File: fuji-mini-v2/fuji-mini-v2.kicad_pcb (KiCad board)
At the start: 2 copper layers, 58.4 x 81.3 mm, 59 parts, among them J1 Micro_SD_Card, J2 AudioJack3_SwitchT, J4 USB_C_Receptacle_USB2.0_14P, SW1 RotaryEncoder_Switch, U1 ESP32-S3, U2 PCM5102A, U3 TPA6110A2DGN, U4 ER_OLEDM0.91_1x-I2C, U5 MCP73831-2-MC, U6 AMS1117-3.3

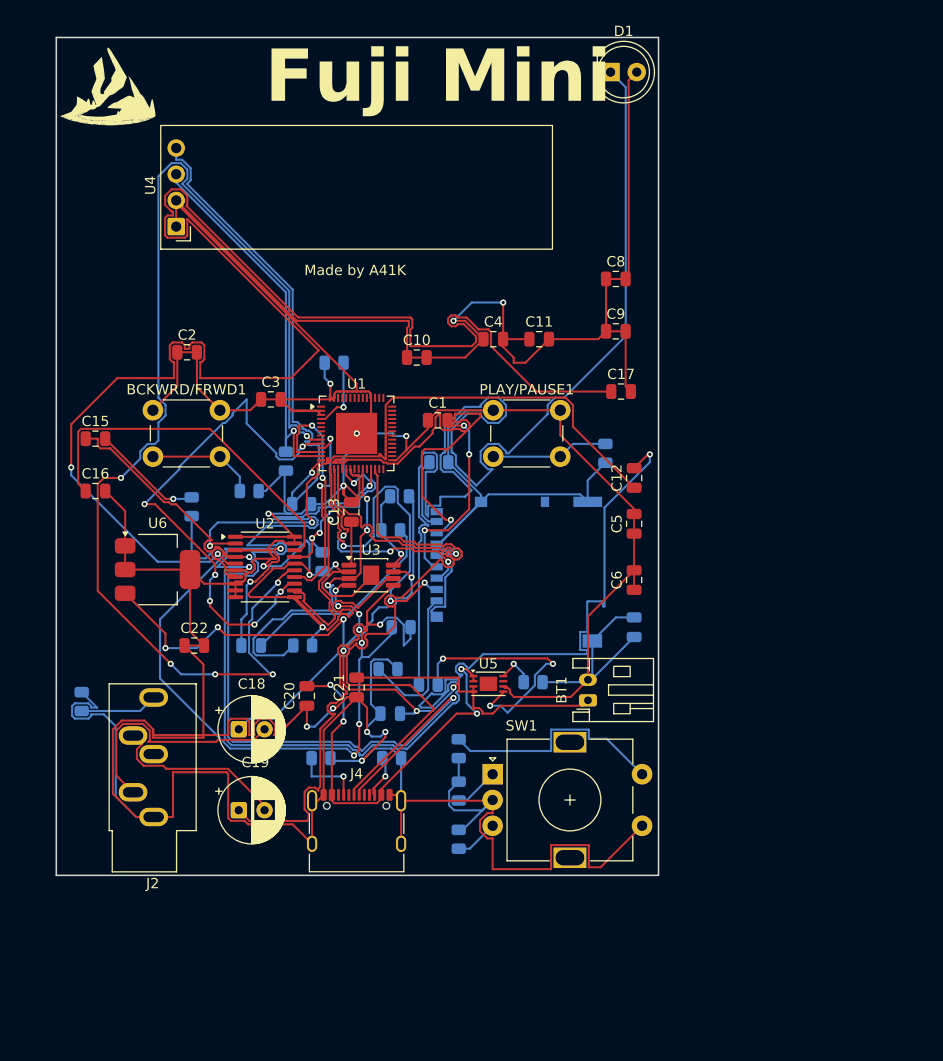
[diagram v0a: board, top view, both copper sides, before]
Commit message: v2.0 2.0 Whole Remake
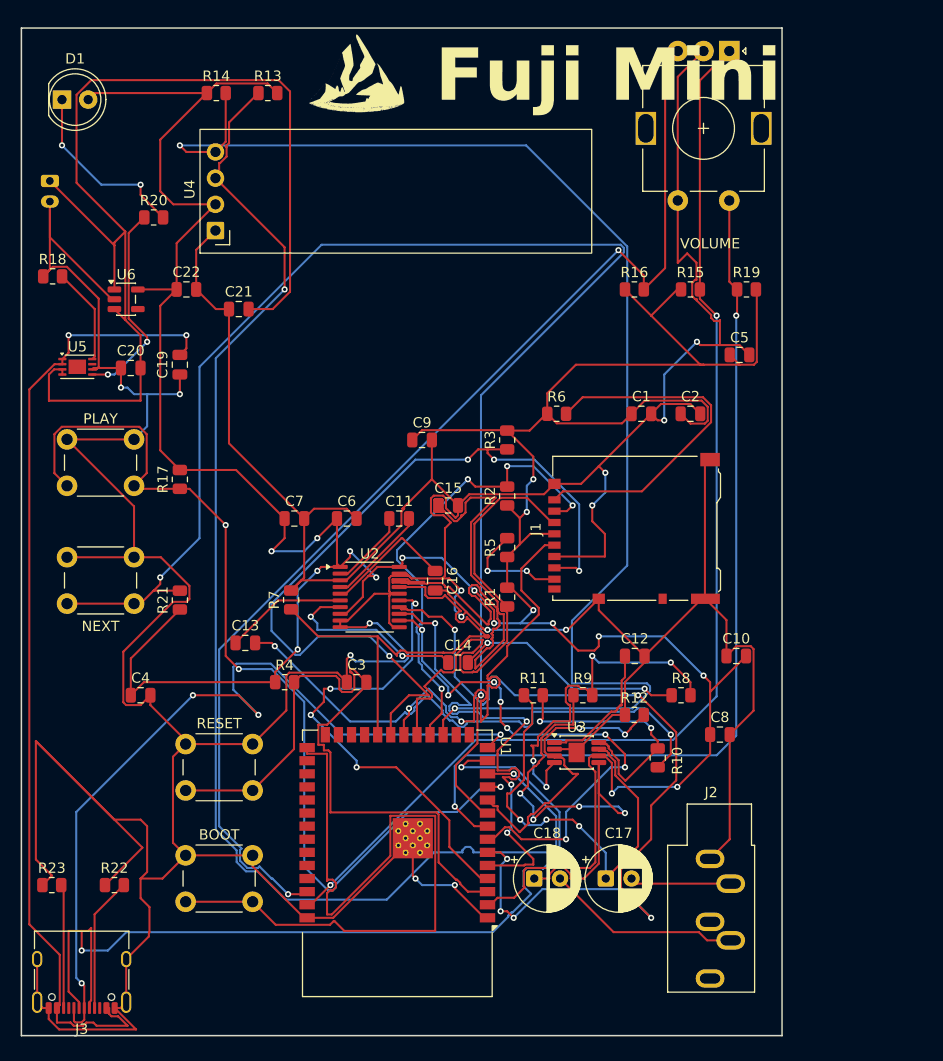
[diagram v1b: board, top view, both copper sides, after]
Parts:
- removed BCKWRD/FRWD1, PLAY/PAUSE1: SW_Push, Button_Switch_THT:SW_PUSH_6mm
- removed C23: 10uF, Capacitor_SMD:C_0805_2012Metric
- removed J4: USB_C_Receptacle_USB2.0_14P, Connector_USB:USB_C_Receptacle_XKB_U262-16XN-4BVC11
- removed SW1: RotaryEncoder_Switch, Rotary_Encoder:RotaryEncoder_Alps_EC11E-Switch_Vertical_H20mm
- added BOOT: SW_Push, Button_Switch_THT:SW_PUSH_6mm, F.Cu at (91.4, 134.9)
- added J3: USB_C, Connector_USB:USB_C_Receptacle_XKB_U262-16XN-4BVC11, F.Cu at (81.3, 146.1)
- added NEXT: SW_Push, Button_Switch_THT:SW_PUSH_6mm, F.Cu at (79.9, 106.0)
- added PLAY: SW_Push, Button_Switch_THT:SW_PUSH_6mm, F.Cu at (79.9, 94.6)
- added R22: 5.1k, Resistor_SMD:R_0805_2012Metric, F.Cu at (84.5, 137.8)
- added R23: 5.1k, Resistor_SMD:R_0805_2012Metric, F.Cu at (78.4, 137.8)
- added RESET: SW_Push, Button_Switch_THT:SW_PUSH_6mm, F.Cu at (91.4, 124.1)
- added VOLUME: RotaryEncoder_Switch, Rotary_Encoder:RotaryEncoder_Alps_EC11E-Switch_Vertical_H20mm, F.Cu at (144.1, 56.9)
- BT1: moved to B.Cu
- C1, C5: value 100nF -> 10uF
- C11, C16: value 100nF -> 2.2uF
- C14, C7, J1, R1, R12, R15, R17, R2, R3, R4, R8, R9: moved to F.Cu
- C15: value 1uF -> 100nF
- C17: value 100nF -> 220uF; footprint Capacitor_SMD:C_0805_2012Metric -> Capacitor_THT:CP_Radial_D6.3mm_P2.50mm
- C19: value 220uF -> 4.7uF; footprint Capacitor_THT:CP_Radial_D6.3mm_P2.50mm -> Capacitor_SMD:C_0805_2012Metric
- C20: value 1uF -> 10uF
- C21, C22: value 10uF -> 1uF
- C3: value 100nF -> 1uF
- R10: value 4.7k -> 20k; moved to F.Cu
- R11: value 4.7k -> 10k; moved to F.Cu
- R13, R14: value 10k -> 4.7k; moved to F.Cu
- R16: value 2k -> 10k; moved to F.Cu
- R18: value 5.1k -> 2k; moved to F.Cu
- R19: value 5.1k -> 10k; moved to F.Cu
- R20: value 10k -> 1k; moved to F.Cu
- R21: value 1k -> 10k; moved to F.Cu
- R5, R6, R7: value 20k -> 10k; moved to F.Cu
- U1: value ESP32-S3 -> ESP32-S3-WROOM-1; footprint Package_DFN_QFN:QFN-56-1EP_7x7mm_P0.4mm_EP4x4mm -> RF_Module:ESP32-S3-WROOM-1
- U6: value AMS1117-3.3 -> AP2112K-3.3; footprint Package_TO_SOT_SMD:SOT-223-3_TabPin2 -> Package_TO_SOT_SMD:SOT-23-5
- moved R13 74.7 mm to (99.3, 61.0), turned to 0 degrees
- moved BT1 72.5 mm to (78.2, 69.5), turned to -90 degrees
- moved R15 71.3 mm to (140.3, 80.0), turned to 0 degrees
- moved R19 57.0 mm to (145.8, 80.0), turned to 0 degrees
- moved J2 54.1 mm to (142.2, 135.3), turned to 0 degrees
- moved R18 53.5 mm to (78.5, 78.7), turned to 0 degrees
- moved D1 53.3 mm to (79.4, 61.6)
- moved R14 51.4 mm to (94.3, 61.0), turned to 0 degrees
- moved U5 50.4 mm to (80.9, 87.5)
- moved C2 49.2 mm to (140.3, 92.1)
- moved C4 48.6 mm to (87.0, 119.4)
- moved C17 47.3 mm to (132.1, 137.2)
- moved R10 46.1 mm to (137.2, 125.5), turned to 90 degrees
- moved C8 45.3 mm to (143.2, 123.2)
- moved C19 43.6 mm to (90.8, 87.3), turned to 90 degrees
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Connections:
- BT1 pad 2: 3V3 -> GND
- C1 pad 1: 3V3 -> +3V3
- C1 pad 2: Net-(J1-VDD) -> GND
- C10 pad 1: 3V3 -> GND
- C10 pad 2: 3V3 -> +3V3
- C11 pad 1: 3V3 -> Net-(U2-CAPP)
- C11 pad 2: 3V3 -> Net-(U2-CAPM)
- C12 pad 1: Net-(U2-CAPP) -> Net-(U3-BYPASS)
- C12 pad 2: Net-(U2-CAPM) -> GND
- C13 pad 1: Net-(U3-BYPASS) -> Net-(U2-OUTL)
- C13 pad 2: 3V3 -> DAC_OUTL
- C14 pad 1: Net-(U2-OUTL) -> Net-(U2-OUTR)
- C14 pad 2: DAC_OUTL -> DAC_OUTR
- C15 pad 1: Net-(U2-OUTR) -> Net-(U2-LDOO)
- C15 pad 2: DAC_OUTR -> GND
- C16 pad 1: Net-(U2-LDOO) -> Net-(U2-VNEG)
- C16 pad 2: 3V3 -> GND
- C17 pad 1: Net-(U2-VNEG) -> VO1
- C17 pad 2: 3V3 -> HP_L
- C18 pad 1: VO1 -> VO2
- C18 pad 2: HP_L -> HP_R
- C19 pad 1: VO2 -> GND
- C19 pad 2: HP_R -> VDD
- C2 pad 1: 3V3 -> +3V3
- C2 pad 2: 3V3 -> GND
- C20 pad 1: 3V3 -> GND
- C20 pad 2: VDD -> VBAT
- C21 pad 1: 3V3 -> GND
- C22 pad 1: 3V3 -> +3V3
- C22 pad 2: 3V3 -> GND
- C3 pad 1: 3V3 -> GND
- C3 pad 2: 3V3 -> Net-(U1-EN)
- C4 pad 1: 3V3 -> +3V3
- C4 pad 2: 3V3 -> GND
- C5 pad 1: 3V3 -> +3V3
- C5 pad 2: 3V3 -> GND
- C6 pad 1: 3V3 -> +3V3
- C6 pad 2: 3V3 -> GND
- C7 pad 1: 3V3 -> +3V3
- C7 pad 2: 3V3 -> GND
- C8 pad 1: 3V3 -> +3V3
- C8 pad 2: 3V3 -> GND
- C9 pad 1: 3V3 -> +3V3
- C9 pad 2: 3V3 -> GND
- D1 pad 2: 3V3 -> +3V3
- J1 pad 4: Net-(J1-VDD) -> +3V3
- J1 pad 6: 3V3 -> GND
- J1 pad SH: 3V3 -> GND
- J2 pad S: 3V3 -> GND
- J2 pad TN: HP_DETECT -> unconnected-(J2-PadTN)
- R1 pad 1: 3V3 -> GPIO11
- R1 pad 2: Net-(J1-DAT2) -> +3V3
- R10 pad 1: I2C_SCL -> DAC_OUTL
- R10 pad 2: 3V3 -> Net-(U3-IN1-)
- R11 pad 1: 3V3 -> VO1
- R11 pad 2: I2C_SDA -> Net-(U3-IN1-)
- R12 pad 1: 3V3 -> GND
- R12 pad 2: ENC_A -> AMP_ENABLE
- R13 pad 1: 3V3 -> I2C_SCL
- R13 pad 2: ENC_B -> +3V3
- R14 pad 1: BTN_PLAY -> +3V3
- R14 pad 2: 3V3 -> I2C_SDA
- R15 pad 1: 3V3 -> +3V3
- R15 pad 2: HP_DETECT -> ENC_A
- R16 pad 1: 3V3 -> +3V3
- R16 pad 2: Net-(U5-PROG) -> ENC_B
- R17 pad 1: Net-(R17-Pad1) -> BTN_PLAY
- R17 pad 2: 3V3 -> +3V3
- R18 pad 1: 3V3 -> GND
- R18 pad 2: Net-(J4-CC1) -> Net-(U5-PROG)
- R19 pad 1: 3V3 -> ENC_BTN
- R19 pad 2: Net-(J4-CC2) -> +3V3
- R2 pad 1: 3V3 -> +3V3
- R2 pad 2: Net-(J1-DAT1) -> GPIO10
- R20 pad 1: 3V3 -> Net-(U5-STAT)
- R20 pad 2: BTN_NEXT -> Net-(D1-K)
- R21 pad 1: Net-(U5-STAT) -> +3V3
- R21 pad 2: Net-(D1-K) -> BTN_NEXT
- R3 pad 1: Net-(U1-CHIP_PU) -> GPIO13
- R3 pad 2: 3V3 -> +3V3
- R4 pad 1: DAC_MUTE -> +3V3
- R4 pad 2: 3V3 -> Net-(U1-EN)
- R5 pad 1: DAC_OUTR -> +3V3
- R5 pad 2: Net-(U3-IN2-) -> Net-(J1-DAT1)
- R6 pad 1: VO2 -> +3V3
- R6 pad 2: Net-(U3-IN2-) -> Net-(J1-DAT2)
- R7 pad 1: DAC_OUTL -> DAC_MUTE
- R7 pad 2: Net-(U3-IN1-) -> GND
- R8 pad 1: VO1 -> DAC_OUTR
- R8 pad 2: Net-(U3-IN1-) -> Net-(U3-IN2-)
- R9 pad 1: 3V3 -> VO2
- R9 pad 2: AMP_ENABLE -> Net-(U3-IN2-)
- U1 pad 1: unconnected-(U1-LNA_IN-Pad1) -> GND
- U1 pad 10: I2S_BCK -> AMP_ENABLE
- U1 pad 11: I2S_DIN -> BTN_PLAY
- U1 pad 12: I2S_SCK -> I2C_SCL
- U1 pad 13: I2C_SCL -> USB_DN
- U1 pad 14: I2C_SDA -> USB_DP
- U1 pad 15: GPIO10 -> unconnected-(U1-IO3-Pad15)
- U1 pad 16: GPIO11 -> unconnected-(U1-IO46-Pad16)
- U1 pad 17: GPIO12 -> I2C_SDA
- U1 pad 18: GPIO13 -> GPIO10
- U1 pad 19: DAC_MUTE -> GPIO11
- U1 pad 2: 3V3 -> +3V3
- U1 pad 20: 3V3 -> GPIO12
- U1 pad 21: unconnected-(U1-XTAL_32K_P-Pad21) -> GPIO13
- U1 pad 22: unconnected-(U1-XTAL_32K_N-Pad22) -> DAC_MUTE
- U1 pad 23: AMP_ENABLE -> unconnected-(U1-IO21-Pad23)
- U1 pad 25: USB_DN -> unconnected-(U1-IO48-Pad25)
- U1 pad 26: USB_DP -> unconnected-(U1-IO45-Pad26)
- U1 pad 27: unconnected-(U1-GPIO21-Pad27) -> Net-(U1-IO0)
- U1 pad 29: 3V3 -> unconnected-(U1-IO36-Pad29)
- U1 pad 3: 3V3 -> Net-(U1-EN)
- U1 pad 38: unconnected-(U1-GPIO33-Pad38) -> ENC_B
- U1 pad 39: unconnected-(U1-GPIO34-Pad39) -> ENC_A
- U1 pad 4: Net-(U1-CHIP_PU) -> I2S_LRCK
- U1 pad 40: unconnected-(U1-GPIO35-Pad40) -> GND
- U1 pad 41: unconnected-(U1-GPIO36-Pad41) -> GND
- U1 pad 5: unconnected-(U1-GPIO0-Pad5) -> I2S_BCK
- U1 pad 6: unconnected-(U1-GPIO1-Pad6) -> I2S_DIN
- U1 pad 7: unconnected-(U1-GPIO2-Pad7) -> I2S_SCK
- U1 pad 8: unconnected-(U1-GPIO3-Pad8) -> ENC_BTN
- U1 pad 9: I2S_LRCK -> BTN_NEXT
- U2 pad 1: 3V3 -> +3V3
- U2 pad 10: 3V3 -> GND
- U2 pad 11: 3V3 -> GND
- U2 pad 16: 3V3 -> GND
- U2 pad 19: 3V3 -> GND
- U2 pad 20: 3V3 -> +3V3
- U2 pad 3: 3V3 -> GND
- U2 pad 8: 3V3 -> +3V3
- U2 pad 9: 3V3 -> GND
- U3 pad 2: 3V3 -> GND
- U3 pad 6: 3V3 -> +3V3
- U3 pad 9: 3V3 -> GND
- U4 pad 1: 3V3 -> GND
- U4 pad 2: 3V3 -> +3V3
- U5 pad 6: 3V3 -> GND
- U6 pad 1: 3V3 -> VBAT
- U6 pad 2: 3V3 -> GND
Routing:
- net 3V3: track 685.5 -> 0.00 mm, vias 16 -> 0
- net GND: track 0.00 -> 596.1 mm, vias 0 -> 14
- net +3V3: track 0.00 -> 353.4 mm, vias 0 -> 17
- net Net-(U2-VNEG): track 151.2 -> 12.8 mm, vias 2 -> 0
- net BTN_NEXT: track 10.6 -> 144.3 mm, vias 0 -> 2
- net ENC_B: track 4.21 -> 113.6 mm, vias 0 -> 2
- net ENC_A: track 4.35 -> 112.6 mm, vias 0 -> 2
- net Net-(D1-K): track 119.7 -> 17.7 mm, vias 0 -> 2
- net Net-(U2-CAPM): track 103.9 -> 9.84 mm, vias 2 -> 0
- net I2C_SCL: track 38.8 -> 129.9 mm, vias 1 -> 2
- net ENC_BTN: track 0.00 -> 88.7 mm, vias 0 -> 2
- net BTN_PLAY: track 11.4 -> 94.8 mm, vias 0 -> 3
- net I2C_SDA: track 49.4 -> 132.7 mm, vias 1 -> 2
- net Net-(U1-IO0): track 0.00 -> 73.0 mm
- net I2S_LRCK: track 115.4 -> 45.9 mm, vias 6 -> 4
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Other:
- board size 58.4 x 81.3 mm -> 73.8 x 97.7 mm
- board text removed: "Made by A41K"
